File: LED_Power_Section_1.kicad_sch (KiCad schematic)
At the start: 60 parts, among them IC2 A6214KLKTR-T, IC3 A6214KLKTR-T, IC4 A6214KLKTR-T, IC5 A6214KLKTR-T, IC6 A6214KLKTR-T, IC7 A6214KLKTR-T

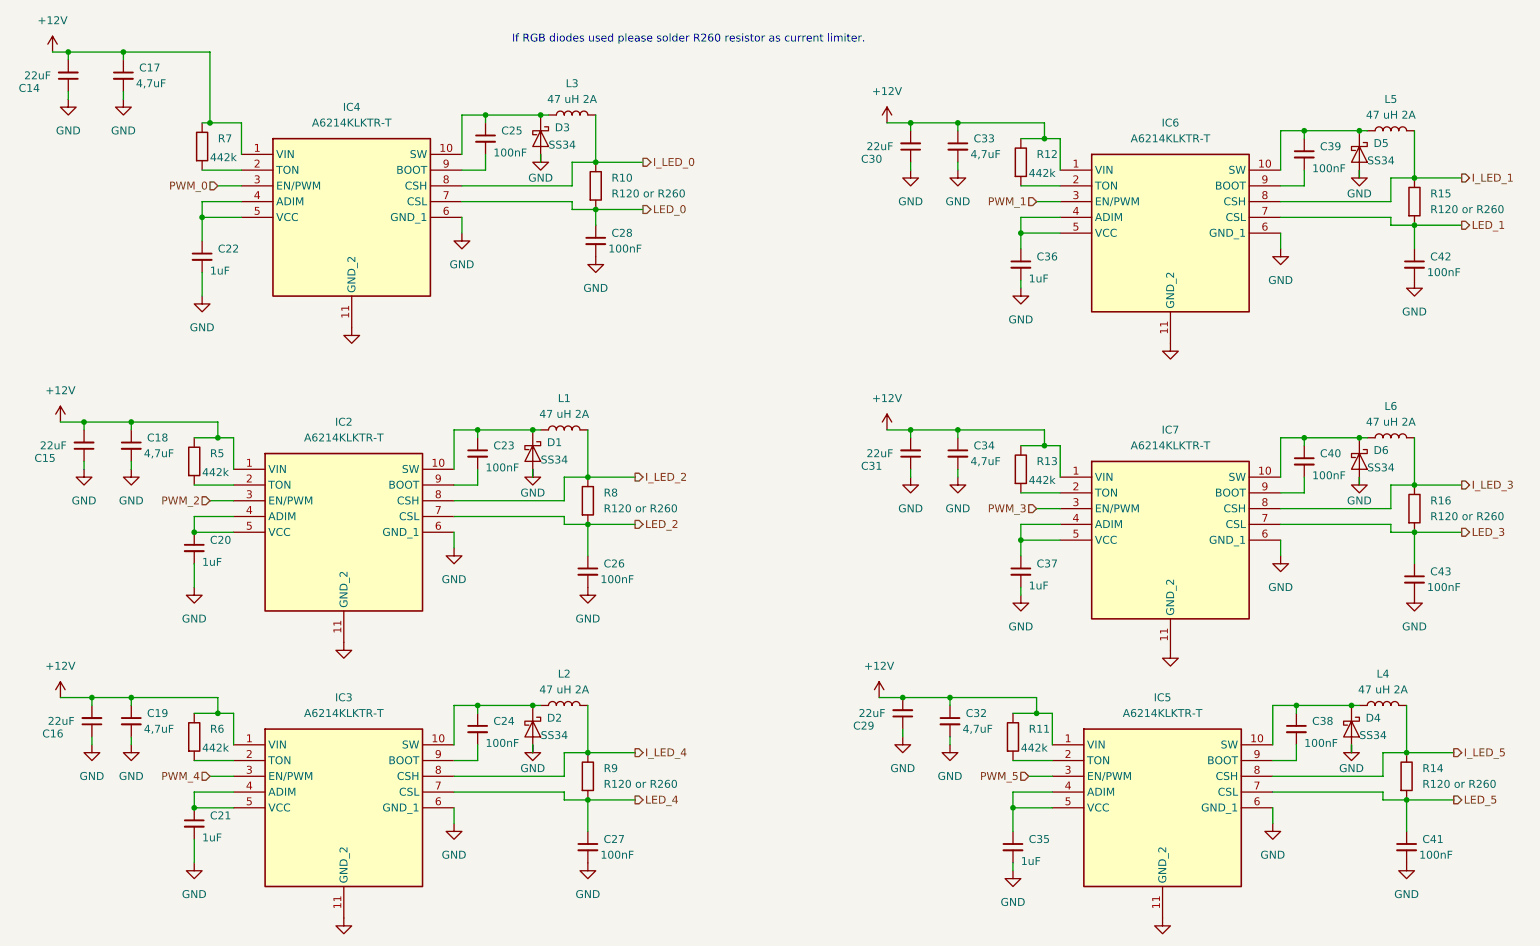
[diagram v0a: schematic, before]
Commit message: wip
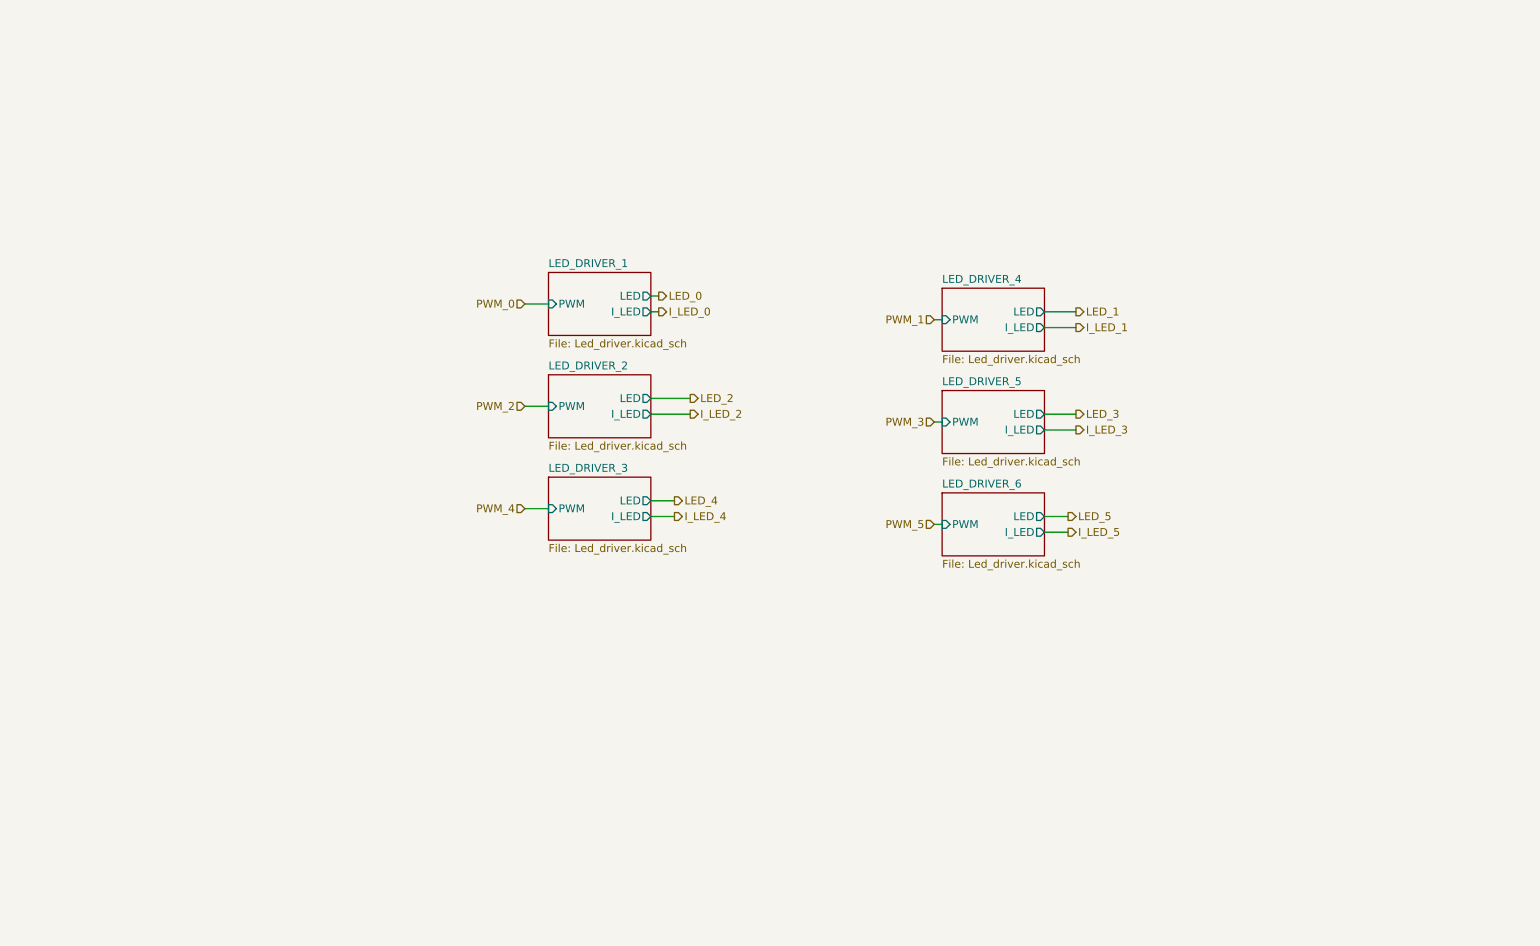
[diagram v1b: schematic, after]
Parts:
- removed C14, C15, C16, C29, C30, C31: 22uF, Capacitor_SMD:C_0805_2012Metric_Pad1.18x1.45mm_HandSolder, symbol Device:C_Small
- removed C17, C18, C19, C32, C33, C34: 4,7uF, Capacitor_SMD:C_0603_1608Metric_Pad1.08x0.95mm_HandSolder, symbol Device:C_Small
- removed C20, C21, C22, C35, C36, C37: 1uF, Capacitor_SMD:C_0603_1608Metric_Pad1.08x0.95mm_HandSolder, symbol Device:C_Small
- removed C23, C24, C25, C26, C27, C28, C38, C39, C40, C41, C42, C43: 100nF, Capacitor_SMD:C_0603_1608Metric_Pad1.08x0.95mm_HandSolder, symbol Device:C_Small
- removed D1, D2, D3, D4, D5, D6: SS34, Diode_SMD:D_SMA, symbol PCM_4ms_Diode:B140-E3
- removed IC2, IC3, IC4, IC5, IC6, IC7: A6214KLKTR-T, LED_Driver:SOP100P600X165-11N, symbol A6214KLKTR-T:A6214KLKTR-T
- removed L1, L2, L3, L4, L5, L6: 47 uH 2A, ADC:CDRH105RNP151NC, symbol Device:L
- removed R10, R14, R15, R16, R8, R9: R120 or R260, Resistor_THT:R_Radial_Power_L16.1mm_W9.0mm_P7.37mm, symbol PCM_SL_Resistors:Resistor
- removed R11, R12, R13, R5, R6, R7: 442k, Resistor_SMD:R_0603_1608Metric_Pad0.98x0.95mm_HandSolder, symbol PCM_SL_Resistors:Resistor
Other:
- added sheet LED_DRIVER_1 (Led_driver.kicad_sch)
- added sheet LED_DRIVER_2 (Led_driver.kicad_sch)
- added sheet LED_DRIVER_3 (Led_driver.kicad_sch)
- added sheet LED_DRIVER_4 (Led_driver.kicad_sch)
- added sheet LED_DRIVER_5 (Led_driver.kicad_sch)
- added sheet LED_DRIVER_6 (Led_driver.kicad_sch)
- note removed: "If RGB diodes used please solder R260 resistor as current limiter."
